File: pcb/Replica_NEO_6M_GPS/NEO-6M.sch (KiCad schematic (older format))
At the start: 9 parts, among them J1 CONUFL001-SMD-T, U2 NEO-6M-GPS

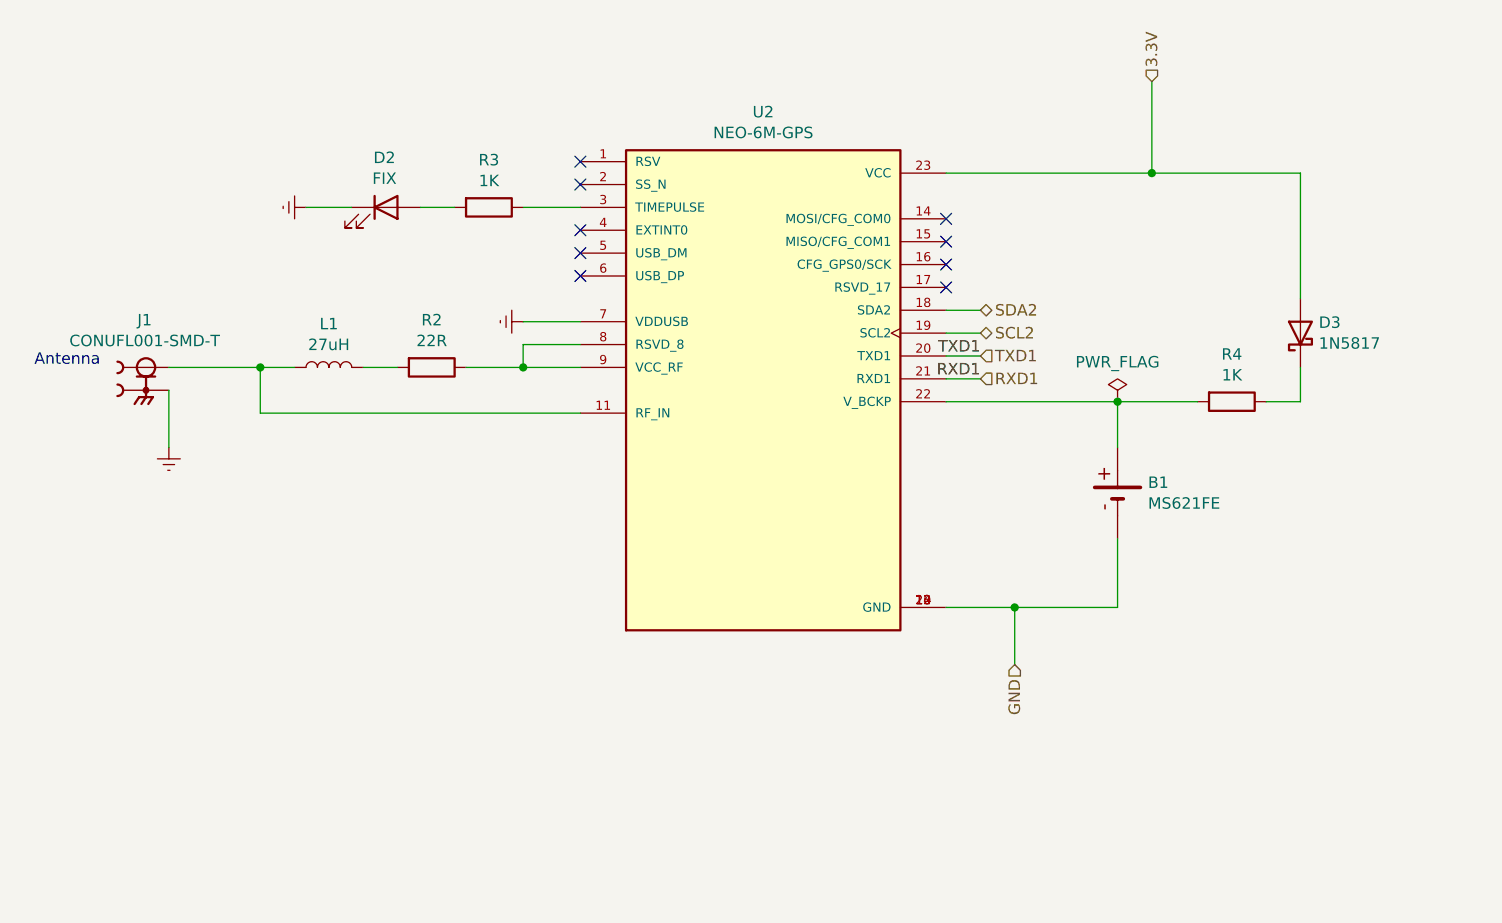
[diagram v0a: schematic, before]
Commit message: se retoco el esquematico
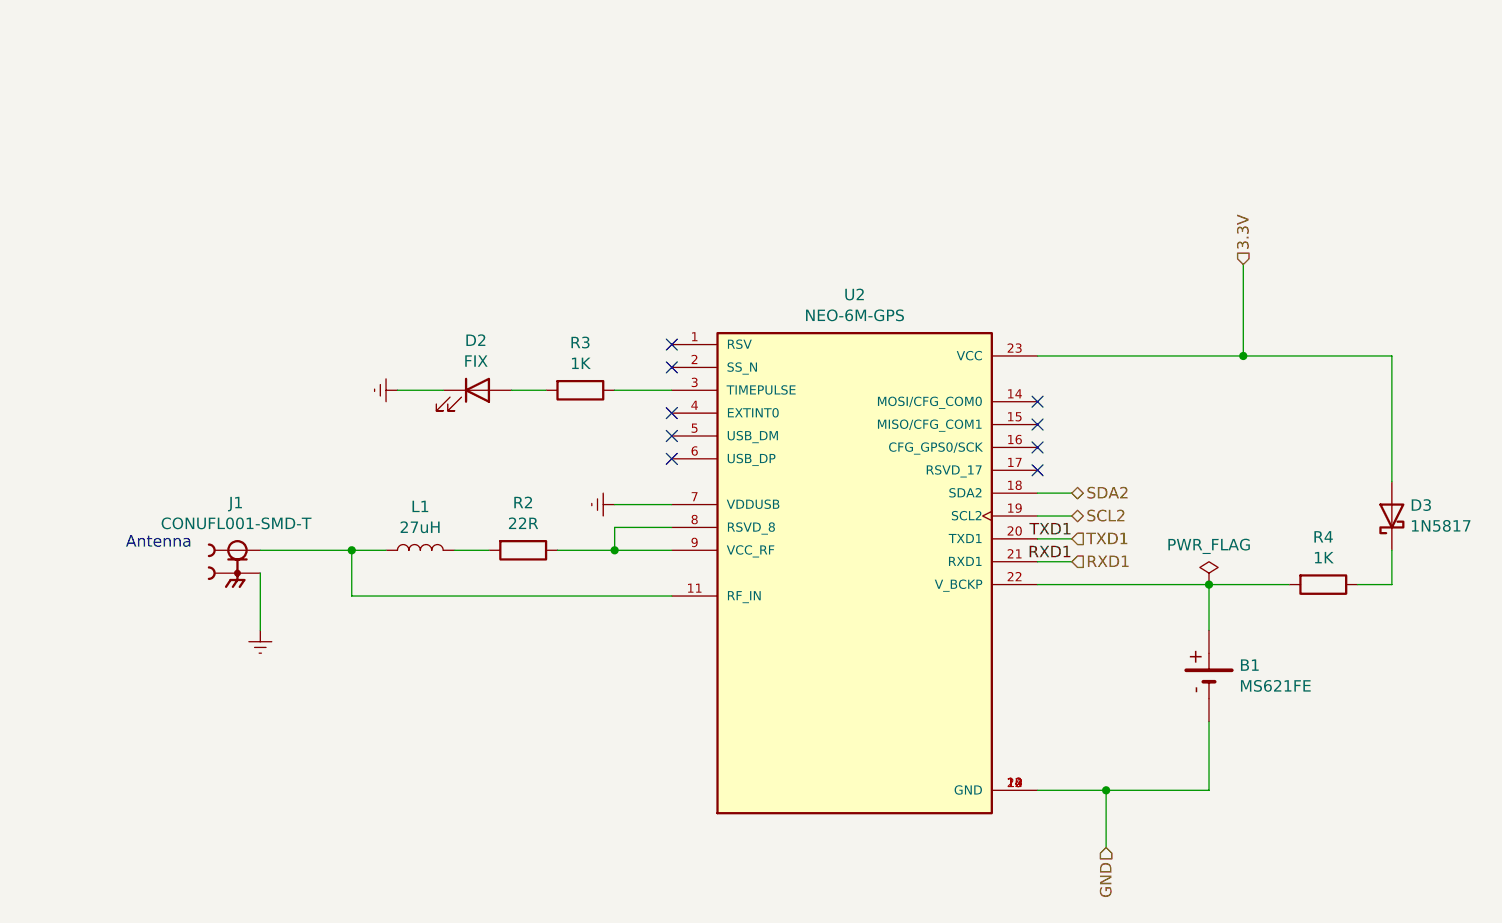
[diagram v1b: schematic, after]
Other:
- moved on the sheet: B1, D2, D3, J1, L1, R2, R3, R4, U2
